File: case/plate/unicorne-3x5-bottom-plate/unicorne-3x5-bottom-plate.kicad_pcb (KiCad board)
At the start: 2 copper layers, 114.8 x 91.4 mm, 6 parts, among them J3 Tenting Puck

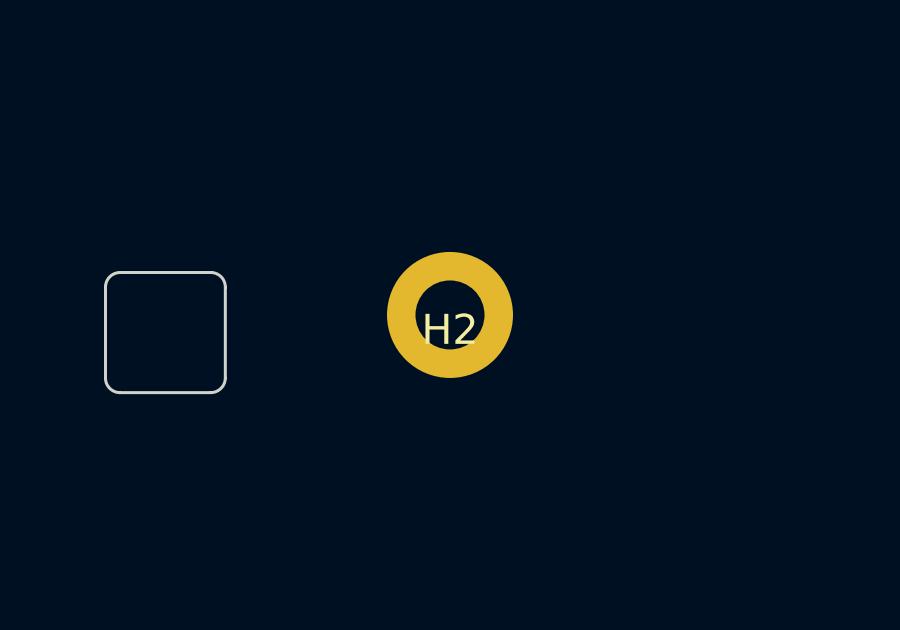
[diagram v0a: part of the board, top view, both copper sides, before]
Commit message: uniCorne 3x6 chocolate
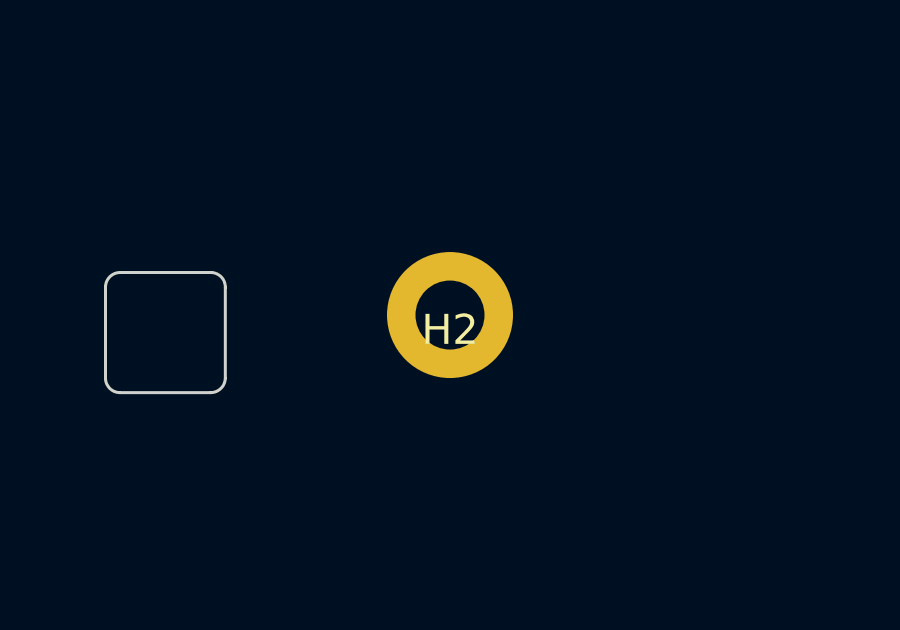
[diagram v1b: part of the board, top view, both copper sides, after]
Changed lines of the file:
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@@
         (effects (font (size 1 1) (thickness 0.15)))
     )
-    (pad "" thru_hole circle locked (at 0 0) (size 4.2 4.2) (drill 2.3) (layers "*.Cu" "*.Mask"))
+    (pad "" thru_hole circle locked (at 0 0.003095) (size 4.2 4.2) (drill 2.3) (layers "*.Cu" "*.Mask"))
   )
   (footprint "KBD_PARTS:M2_Hole_TH" locked (layer "F.Cu")
